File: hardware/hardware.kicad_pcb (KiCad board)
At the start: 2 copper layers, 49.6 x 31.8 mm, 21 parts

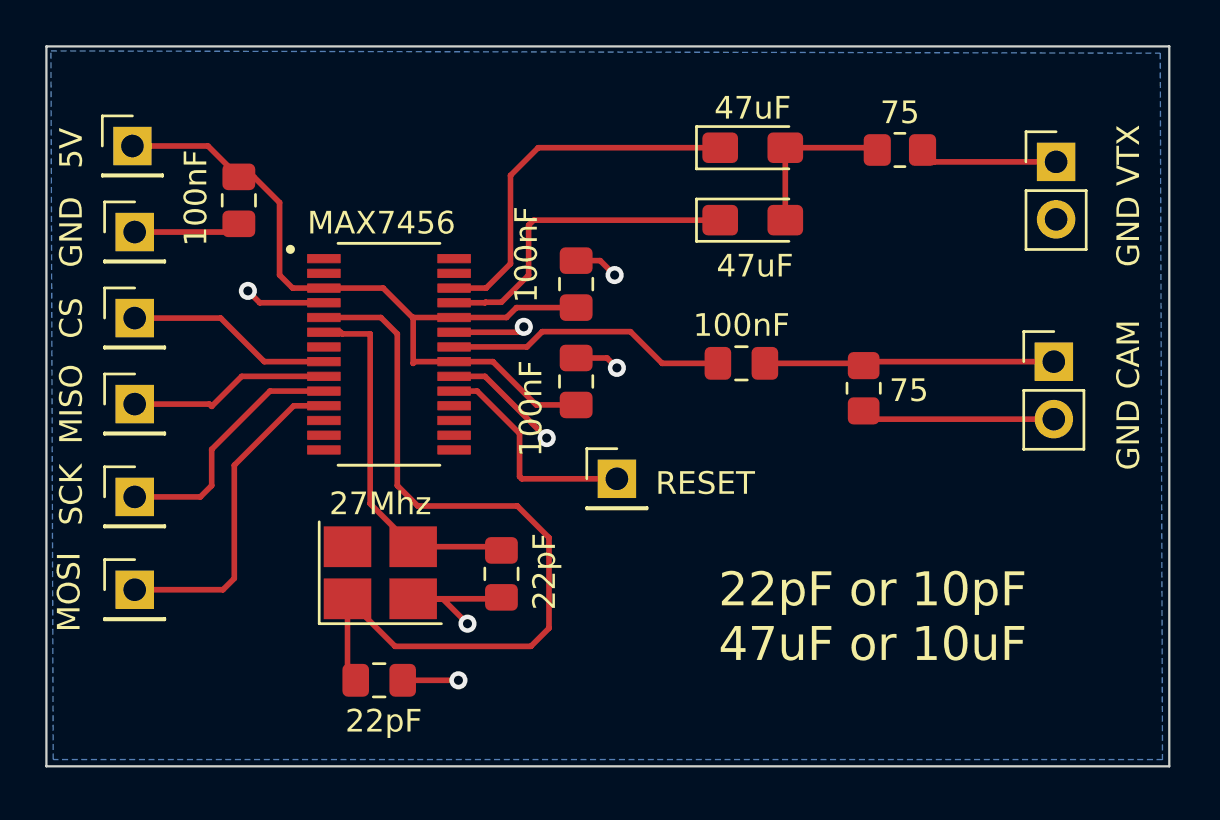
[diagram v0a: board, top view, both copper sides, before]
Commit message: redesign
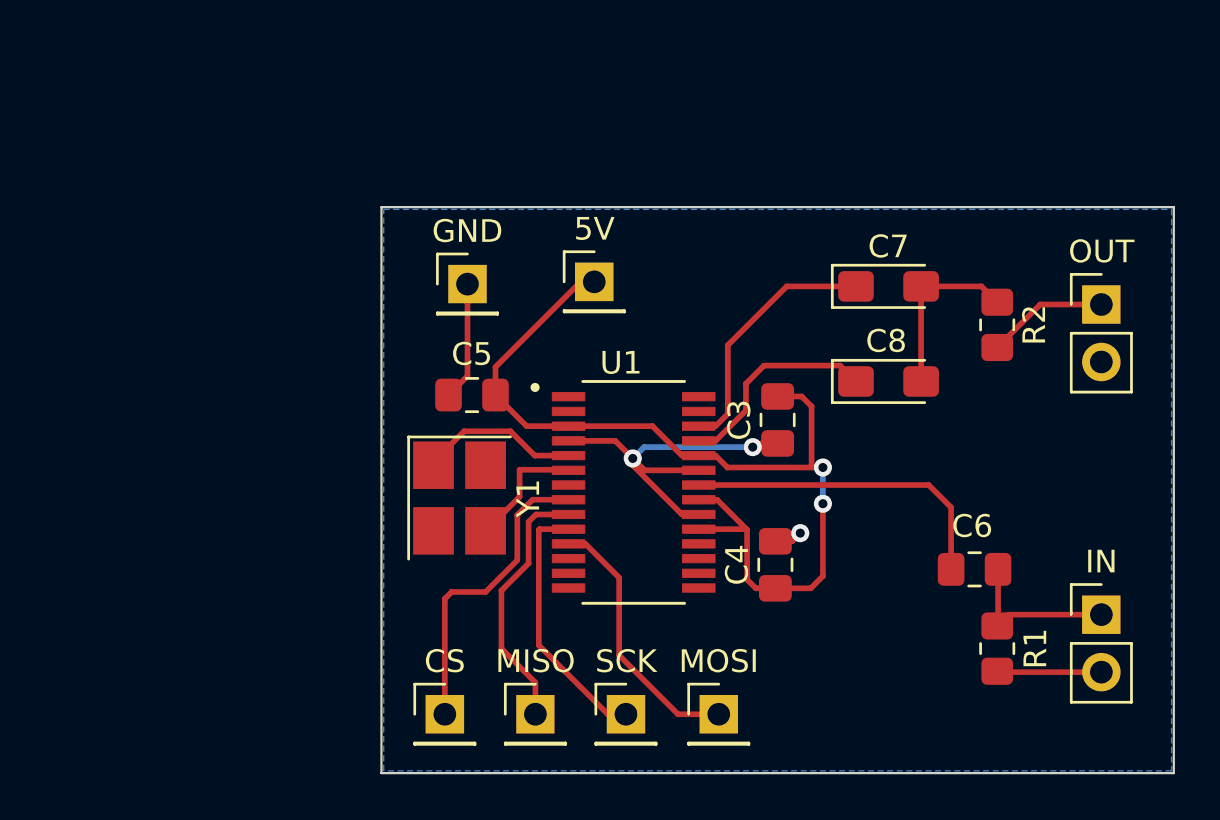
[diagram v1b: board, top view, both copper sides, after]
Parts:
- removed 100nF (x4): 100nF, Capacitor_SMD:C_0805_2012Metric_Pad1.18x1.45mm_HandSolder
- removed 22pF (x2): 22pF, Capacitor_SMD:C_0805_2012Metric_Pad1.18x1.45mm_HandSolder
- removed 27Mhz: Resonator, Crystal:Crystal_SMD_3225-4Pin_3.2x2.5mm_HandSoldering
- removed 47uF (x2): 47uF, Capacitor_Tantalum_SMD:CP_EIA-3216-18_Kemet-A_Pad1.58x1.35mm_HandSolder
- removed 75 (x2): 75, Resistor_SMD:R_0805_2012Metric_Pad1.20x1.40mm_HandSolder
- removed GND CAM: VIN, Connector_PinHeader_2.54mm:PinHeader_1x02_P2.54mm_Vertical
- removed GND VTX: VOUT, Connector_PinHeader_2.54mm:PinHeader_1x02_P2.54mm_Vertical
- removed MAX7456: MAX7456EUI+, MAX7456:SOP65P637X110-28N
- removed RESET: RESET, Connector_PinHeader_2.54mm:PinHeader_1x01_P2.54mm_Vertical
- added C3: 100nF, Capacitor_SMD:C_0805_2012Metric_Pad1.18x1.45mm_HandSolder, F.Cu at (157.0, 86.2)
- added C4: 100nF, Capacitor_SMD:C_0805_2012Metric_Pad1.18x1.45mm_HandSolder, F.Cu at (156.9, 92.6)
- added C5: 100nF, Capacitor_SMD:C_0805_2012Metric_Pad1.18x1.45mm_HandSolder, F.Cu at (143.5, 85.1)
- added C6: 100nF, Capacitor_SMD:C_0805_2012Metric_Pad1.18x1.45mm_HandSolder, F.Cu at (165.7, 92.8)
- added C7: 47uF, Capacitor_Tantalum_SMD:CP_EIA-3216-18_Kemet-A_Pad1.58x1.35mm_HandSolder, F.Cu at (161.9, 80.3)
- added C8: 47uF, Capacitor_Tantalum_SMD:CP_EIA-3216-18_Kemet-A_Pad1.58x1.35mm_HandSolder, F.Cu at (161.9, 84.5)
- added IN: VIN, Connector_PinHeader_2.54mm:PinHeader_1x02_P2.54mm_Vertical, F.Cu at (171.3, 94.8)
- added OUT: VOUT, Connector_PinHeader_2.54mm:PinHeader_1x02_P2.54mm_Vertical, F.Cu at (171.3, 81.1)
- added R1: 75, Resistor_SMD:R_0805_2012Metric_Pad1.20x1.40mm_HandSolder, F.Cu at (166.7, 96.3)
- added R2: 75, Resistor_SMD:R_0805_2012Metric_Pad1.20x1.40mm_HandSolder, F.Cu at (166.7, 82.0)
- added U1: MAX7456EUI+, MAX7456:SOP65P637X110-28N, F.Cu at (150.6, 89.4)
- added Y1: 27MHZ, Crystal:Crystal_SMD_3225-4Pin_3.2x2.5mm_HandSoldering, F.Cu at (142.9, 89.7)
- moved MOSI 26.4 mm to (154.4, 99.2)
- moved SCK 23.7 mm to (150.3, 99.2)
- moved MISO 22.4 mm to (146.3, 99.2)
- moved CS 22.2 mm to (142.3, 99.2)
- moved 5V 21.3 mm to (148.9, 80.1)
- moved GND 14.9 mm to (143.3, 80.2)
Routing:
- net XTAL1: track 35.7 -> 7.12 mm
- net Net-(C6-Pad2): track 12.9 -> 0.00 mm
- net XTAL2: track 16.2 -> 5.50 mm
- net GND: track 38.5 -> 28.2 mm, vias 7 -> 3
- net RESET: track 9.91 -> 0.00 mm
- net 5V: track 34.8 -> 42.9 mm, vias 0 -> 2
- net Net-(J8-Pin_1): track 0.00 -> 7.32 mm
- net Net-(J9-Pad1): track 6.12 -> 0.00 mm
- net Net-(J9-Pin_1): track 0.00 -> 5.39 mm
- net VOUT: track 16.6 -> 11.3 mm
- net SAG: track 14.6 -> 9.31 mm
- net CS: track 9.15 -> 13.5 mm
- net MOSI: track 14.7 -> 11.8 mm
- net MISO: track 8.95 -> 11.5 mm
- net VIN: track 12.5 -> 14.3 mm
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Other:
- board size 49.6 x 31.8 mm -> 35 x 25 mm
- board text removed: "22pF or 10pF 47uF or 10uF"
